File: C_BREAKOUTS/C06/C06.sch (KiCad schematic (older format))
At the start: 40 parts, among them J1 Conn_01x02_Female, J10 Conn_01x02_Female, J11 Conn_01x02_Female, J12 Conn_01x02_Female, J13 Conn_01x02_Female, J14 Conn_01x02_Female, J15 Conn_01x02_Female, J16 Conn_01x02_Female, J17 Conn_01x02_Female, J18 Conn_01x02_Female, J19 Conn_01x02_Female, J2 Conn_01x02_Female, J20 Conn_01x02_Female, J21 Conn_01x02_Female, J22 Conn_01x02_Female, J23 Conn_01x02_Female, J24 Conn_01x02_Female, J25 Conn_01x02_Female, J26 Conn_01x02_Female, J27 Conn_01x04_Female, J28 Conn_01x04_Female, J29 Conn_01x04_Female, J3 Conn_01x02_Female, J30 Conn_01x04_Female, J31 Conn_01x04_Female, J32 Conn_01x04_Female, J33 Conn_01x04_Female, J34 Conn_01x04_Female, J35 Conn_01x04_Female, J36 Conn_01x04_Female, J4 Conn_01x07_Female, J5 Conn_01x07_Female, J6 Conn_01x02_Female, J7 Conn_01x09_Female, J8 Conn_01x09_Female, J9 Conn_01x02_Female

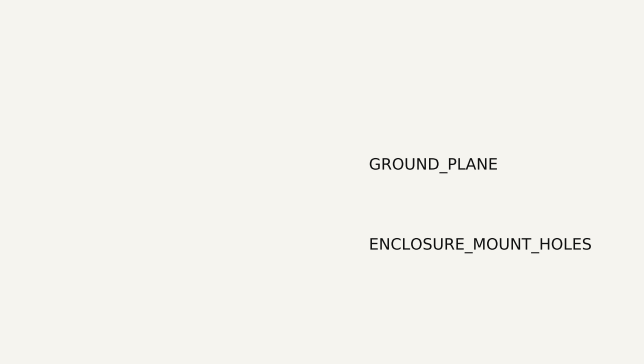
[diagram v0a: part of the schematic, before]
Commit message: single gerber
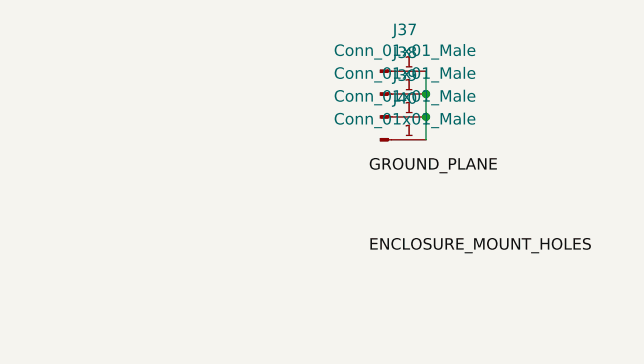
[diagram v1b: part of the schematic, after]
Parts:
- added J37, J38, J39, J40: Conn_01x01_Male, Connector_Wire:SolderWirePad_1x01_Drill1mm, symbol Connector:Conn_01x01_Male
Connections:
- new net: J37.1 (Pin_1), J38.1 (Pin_1), J39.1 (Pin_1), J40.1 (Pin_1)
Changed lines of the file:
@@
 	6200 3600 6200 3700
 Connection ~ 6200 3600
+$Comp
+L Connector:Conn_01x01_Male J37
+U 1 1 5F65D4D3
+P 9900 700
+F 0 "J37" H 10008 881 50  0000 C CNN
+F 1 "Conn_01x01_Male" H 10008 790 50  0000 C CNN
+F 2 "Connector_Wire:SolderWirePad_1x01_Drill1mm" H 9900 700 50  0001 C CNN
+F 3 "~" H 9900 700 50  0001 C CNN
+	1    9900 700
+	1    0    0    -1
+$EndComp
+$Comp
+L Connector:Conn_01x01_Male J38
+U 1 1 5F65E061
+P 9900 800
+F 0 "J38" H 10008 981 50  0000 C CNN
+F 1 "Conn_01x01_Male" H 10008 890 50  0000 C CNN
+F 2 "Connector_Wire:SolderWirePad_1x01_Drill1mm" H 9900 800 50  0001 C CNN
+F 3 "~" H 9900 800 50  0001 C CNN
+	1    9900 800
+	1    0    0    -1
+$EndComp
+$Comp
+L Connector:Conn_01x01_Male J39
+U 1 1 5F65F34A
+P 9900 900
+F 0 "J39" H 10008 1081 50  0000 C CNN
+F 1 "Conn_01x01_Male" H 10008 990 50  0000 C CNN
+F 2 "Connector_Wire:SolderWirePad_1x01_Drill1mm" H 9900 900 50  0001 C CNN
+F 3 "~" H 9900 900 50  0001 C CNN
+	1    9900 900
+	1    0    0    -1
+$EndComp
+$Comp
+L Connector:Conn_01x01_Male J40
+U 1 1 5F660241
+P 9900 1000
+F 0 "J40" H 10008 1181 50  0000 C CNN
+F 1 "Conn_01x01_Male" H 10008 1090 50  0000 C CNN
+F 2 "Connector_Wire:SolderWirePad_1x01_Drill1mm" H 9900 1000 50  0001 C CNN
+F 3 "~" H 9900 1000 50  0001 C CNN
+	1    9900 1000
+	1    0    0    -1
+$EndComp
+Wire Wire Line
+	10100 700  10100 800
+Wire Wire Line
+	10100 800  10100 900
+Connection ~ 10100 800
+Wire Wire Line
+	10100 900  10100 1000
+Connection ~ 10100 900
 $EndSCHEMATC
